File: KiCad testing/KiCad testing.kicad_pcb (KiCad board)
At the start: 2 copper layers, 101.6 x 127 mm, 37 parts, among them J1 USB_A, Q1 IRF540N, Q2 IRF540N, Q3 IRF540N, U1 IR2213, U3 ACS712xLCTR-05B, U4 IR2213

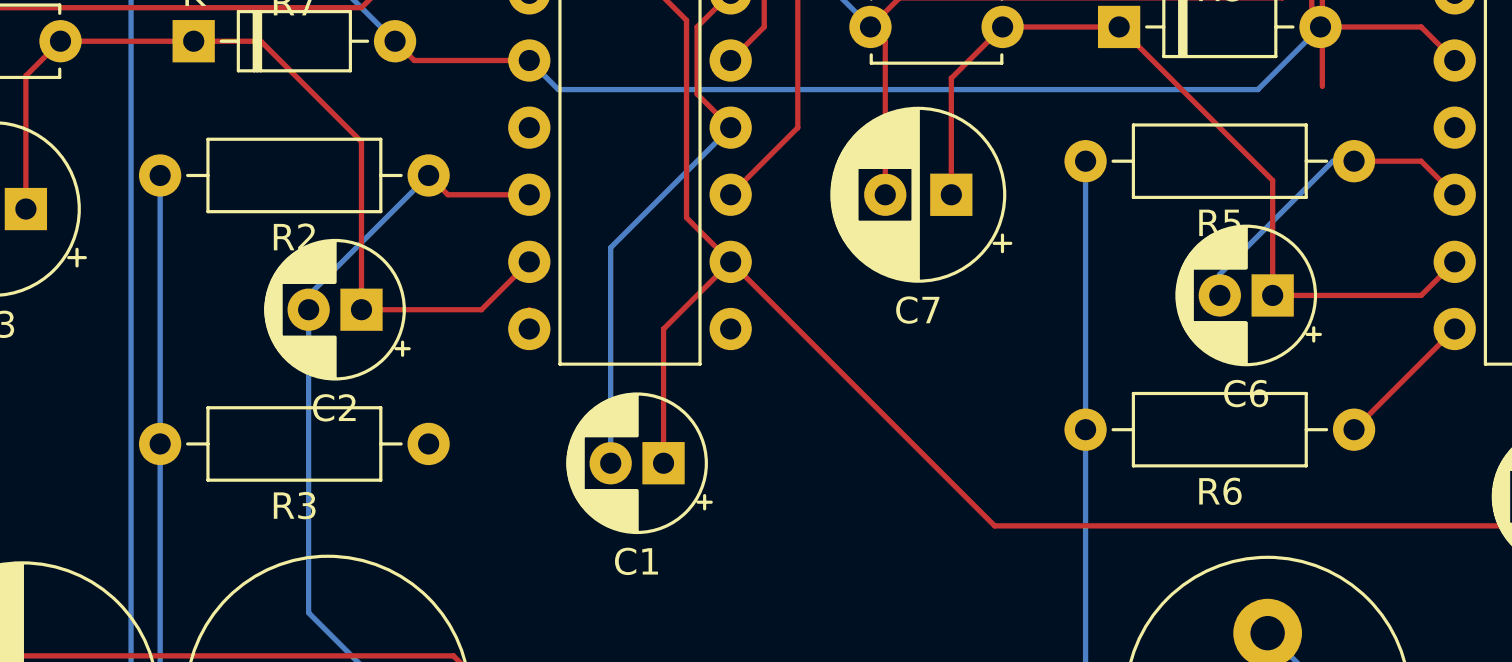
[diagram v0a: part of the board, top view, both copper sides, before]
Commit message: Update Schematic
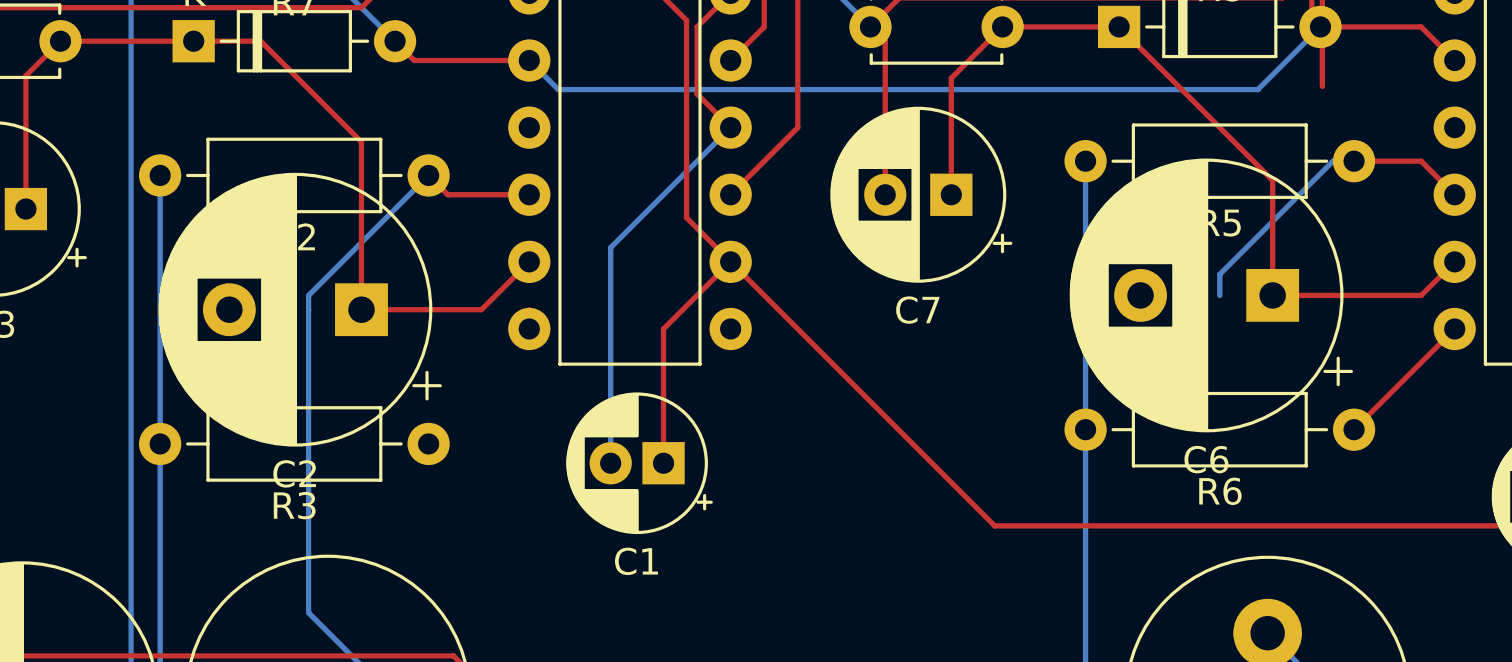
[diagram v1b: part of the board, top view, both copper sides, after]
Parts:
- C2, C6: value 10uF -> 470uF; footprint Capacitor_THT:CP_Radial_D5.0mm_P2.00mm -> Capacitor_THT:CP_Radial_D10.0mm_P5.00mm
